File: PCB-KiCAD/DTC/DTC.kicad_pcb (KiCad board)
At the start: 2 copper layers, 16 parts, among them J1 Conn_01x14, J2 Conn_01x02, J3 Conn_01x02, J4 PJ-102A, J5 Screw_Terminal_01x03, K1 G5LE-1, Q1 BC337, Q2 BC327, U1 NodeMCU1.0(ESP-12E)

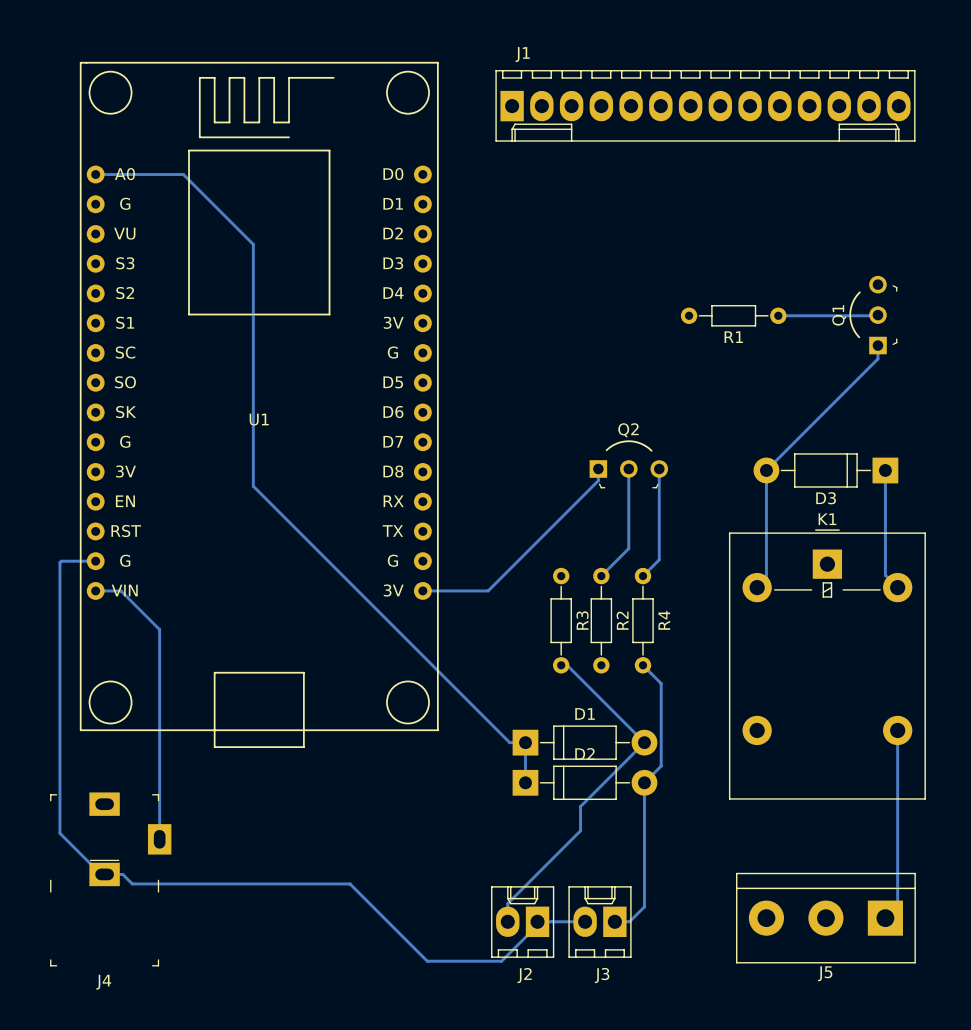
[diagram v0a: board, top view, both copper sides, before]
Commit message: Updated PCB
Updated PCB and added pdf's of layers
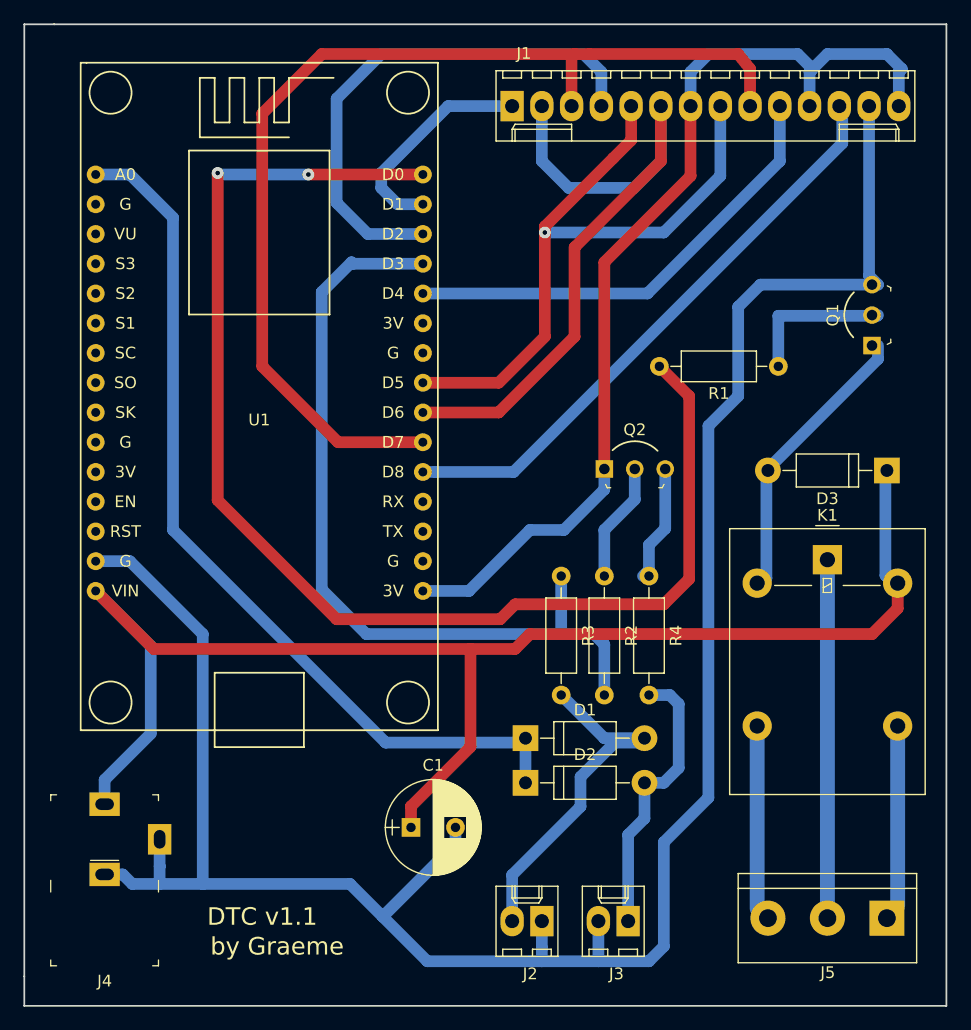
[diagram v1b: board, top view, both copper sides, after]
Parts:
- added C1: 100uF, Capacitors_ThroughHole:CP_Radial_D8.0mm_P3.80mm, F.Cu at (132.1, 127.0)
- R1, R2, R3, R4: footprint Resistors_ThroughHole:R_Axial_DIN0204_L3.6mm_D1.6mm_P7.62mm_Horizontal -> Resistors_ThroughHole:R_Axial_DIN0207_L6.3mm_D2.5mm_P10.16mm_Horizontal
- moved R1 4.32 mm to (163.4, 87.6)
- moved J3 1.13 mm to (150.6, 135.0)
- moved Q1 0.51 mm to (171.4, 85.9)
- moved Q2 0.51 mm to (148.6, 96.4)
- moved R4 0.51 mm to (152.4, 105.5)
- moved D1 0.38 mm to (141.9, 119.4)
- moved K1 0.38 mm to (167.6, 104.1)
- moved J2 0.37 mm to (143.3, 135.0)
- moved R2 0.25 mm to (148.6, 105.5)
- moved D3 0.13 mm to (172.7, 96.5)
- moved J5 0.13 mm to (172.7, 134.7)
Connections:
- D3 pad 1: Net-(D3-Pad1) -> Net-(C1-Pad1)
- J1 pad 13: Net-(J1-Pad13) -> Net-(C1-Pad2)
- J2 pad 1: Net-(J2-Pad1) -> Net-(C1-Pad2)
- J3 pad 2: Net-(J2-Pad1) -> Net-(C1-Pad2)
- J4 pad 1: Net-(J4-Pad1) -> Net-(C1-Pad1)
- J4 pad 2: Net-(J2-Pad1) -> Net-(C1-Pad2)
- J4 pad 3: Net-(D3-Pad1) -> Net-(C1-Pad2)
- K1 pad 1: Net-(J5-Pad3) -> Net-(J5-Pad2)
- K1 pad 3: Net-(J5-Pad2) -> Net-(J5-Pad3)
- K1 pad 5: Net-(D3-Pad1) -> Net-(C1-Pad1)
- Q1 pad 3: Net-(Q1-Pad3) -> Net-(C1-Pad2)
- U1 pad 14: Net-(J2-Pad1) -> Net-(C1-Pad2)
- U1 pad 15: Net-(D3-Pad1) -> Net-(C1-Pad1)
- U1 pad 17: Net-(J1-Pad13) -> Net-(C1-Pad2)
- U1 pad 24: Net-(Q1-Pad3) -> Net-(C1-Pad2)
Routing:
- net Net-(C1-Pad2): track 0.00 -> 191.4 mm
- net Net-(C1-Pad1): track 0.00 -> 123.3 mm
- net Net-(R1-Pad2): track 0.00 -> 110.6 mm, vias 0 -> 2
- net Net-(J1-Pad3): track 0.00 -> 90.1 mm
- net Net-(J2-Pad1): track 77.2 -> 0.00 mm
- net Net-(R2-Pad2): track 0.00 -> 70.6 mm
- net Net-(J1-Pad11): track 19.9 -> 84.4 mm
- net Net-(J1-Pad2): track 0.00 -> 59.8 mm
- net Net-(J1-Pad5): track 0.00 -> 58.5 mm, vias 0 -> 1
- net Net-(J1-Pad12): track 0.00 -> 50.7 mm
- net Net-(J1-Pad4): track 0.00 -> 45.1 mm
- net Net-(J1-Pad10): track 0.00 -> 39.9 mm
- net Net-(D3-Pad1): track 35.2 -> 0.00 mm
- net Net-(J5-Pad2): track 0.00 -> 30.3 mm
- net Net-(J1-Pad1): track 0.00 -> 18.9 mm
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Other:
- board outline added: 78.7 x 83.8 mm
- net class Default: trace_width 0.25 -> 1; via_dia 0.8 -> 1
- board text added: "DTC v1.1"
- board text added: "by Graeme"
